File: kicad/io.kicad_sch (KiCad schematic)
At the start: 20 parts, among them J4 DE9_Plug_MountingHoles, J5 DB25_Receptacle_MountingHoles, U29 6522, U30 6551, U31 6551, U32 MAX232, U34 24LC256, X2 ACO-1.8432MHz-A

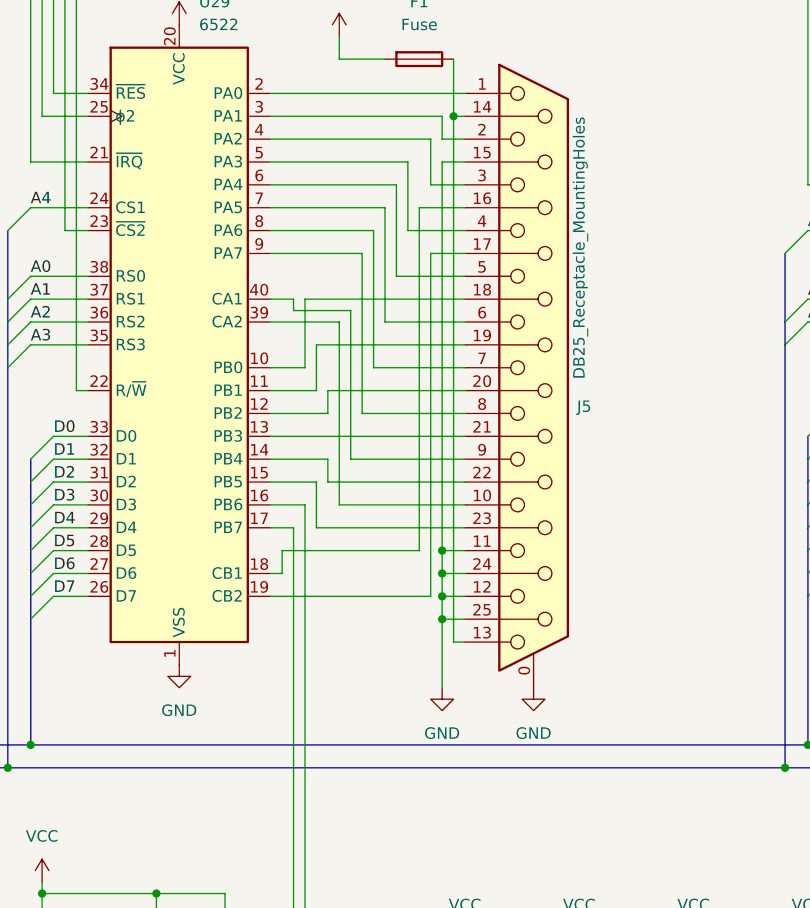
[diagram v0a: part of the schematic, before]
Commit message: Bugfixes, start routing
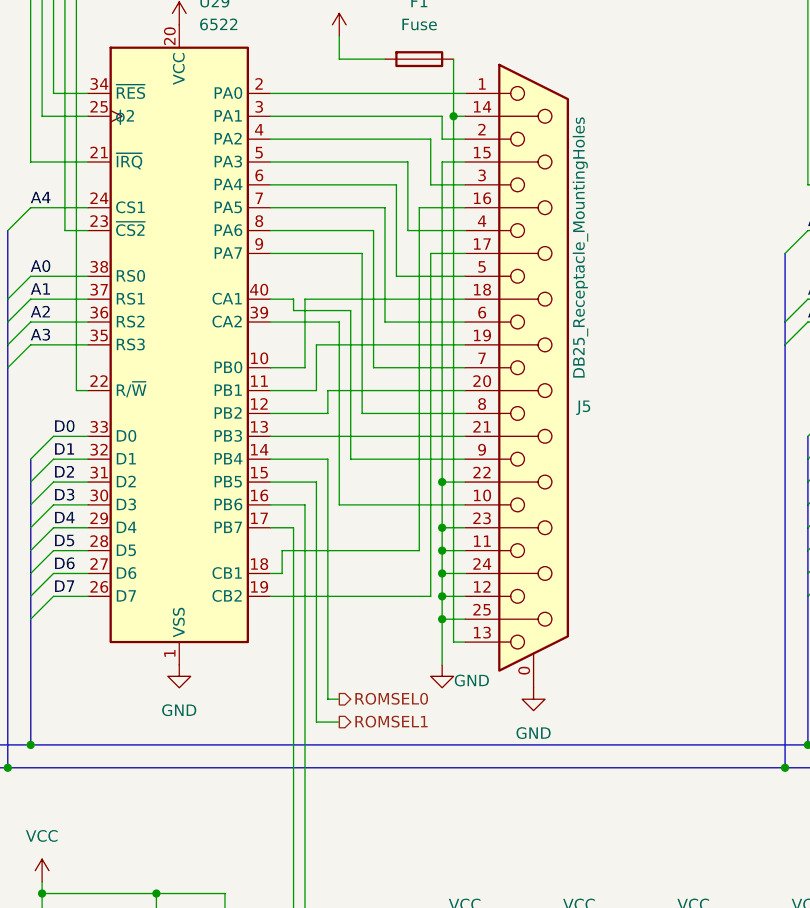
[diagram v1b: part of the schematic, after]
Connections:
- net GND: now also J5.22 (P22), J5.23 (P23)
- net ROMSEL0: now reaches U29.14 (PB4)
- net ROMSEL0: no longer J5.22 (P22)
- net ROMSEL1: now reaches U29.15 (PB5)
- net ROMSEL1: no longer J5.23 (P23)
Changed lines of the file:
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@@
 	)
 	(junction
+		(at 80.01 97.79)
+		(diameter 0)
+		(color 0 0 0 0)
+	)
+	(junction
 		(at 242.57 26.67)
 		(diameter 0)
@@
 	)
 	(junction
+		(at 80.01 92.71)
+		(diameter 0)
+		(color 0 0 0 0)
+	)
+	(junction
 		(at 35.56 138.43)
 		(diameter 0)
@@
 	(wire
 		(pts
+			(xy 80.01 97.79) (xy 80.01 92.71)
+		)
+		(stroke
+			(width 0)
+			(type default)
+		)
+	)
+	(wire
+		(pts
 			(xy 137.16 114.3) (xy 148.59 114.3)
 		)
@@
 	(wire
 		(pts
-			(xy 66.04 92.71) (xy 66.04 97.79)
+			(xy 66.04 92.71) (xy 66.04 119.38)
 		)
 		(stroke
@@
 	(wire
 		(pts
+			(xy 80.01 97.79) (xy 82.55 97.79)
+		)
+		(stroke
+			(width 0)
+			(type default)
+		)
+	)
+	(wire
+		(pts
 			(xy 35.56 162.56) (xy 24.13 162.56)
 		)
@@
 	(wire
 		(pts
+			(xy 80.01 92.71) (xy 82.55 92.71)
+		)
+		(stroke
+			(width 0)
+			(type default)
+		)
+	)
+	(wire
+		(pts
 			(xy 63.5 73.66) (xy 69.85 73.66)
 		)
@@
 		)
 	)
+	(wire
+		(pts
+			(xy 66.04 119.38) (xy 68.58 119.38)
+		)
+		(stroke
+			(width 0)
+			(type default)
+		)
+	)
 	(bus
 		(pts
@@
 	(wire
 		(pts
+			(xy 67.31 116.84) (xy 68.58 116.84)
+		)
+		(stroke
+			(width 0)
+			(type default)
+		)
+	)
+	(wire
+		(pts
 			(xy 265.43 128.27) (xy 262.89 128.27)
 		)
@@
 	(wire
 		(pts
-			(xy 66.04 97.79) (xy 82.55 97.79)
-		)
-		(stroke
-			(width 0)
-			(type default)
-		)
-	)
-	(wire
-		(pts
 			(xy 255.27 154.94) (xy 265.43 154.94)
 		)
@@
 		)
 	)
-	(wire
-		(pts
-			(xy 67.31 92.71) (xy 82.55 92.71)
-		)
-		(stroke
-			(width 0)
-			(type default)
-		)
-	)
 	(bus
 		(pts
@@
 	(wire
 		(pts
-			(xy 80.01 115.57) (xy 80.01 107.95)
+			(xy 80.01 113.03) (xy 80.01 107.95)
 		)
 		(stroke
@@
 	(wire
 		(pts
+			(xy 80.01 92.71) (xy 80.01 57.15)
+		)
+		(stroke
+			(width 0)
+			(type default)
+		)
+	)
+	(wire
+		(pts
 			(xy 209.55 104.14) (xy 222.25 104.14)
 		)
@@
 	(wire
 		(pts
-			(xy 80.01 100.33) (xy 80.01 57.15)
+			(xy 80.01 100.33) (xy 80.01 97.79)
 		)
 		(stroke
@@
 		)
 	)
-	(bus
+	(wire
 		(pts
-			(xy 34.29 95.25) (xy 34.29 97.79)
+			(xy 67.31 90.17) (xy 67.31 116.84)
 		)
 		(stroke
@@
 		)
 	)
-	(wire
+	(bus
 		(pts
-			(xy 67.31 90.17) (xy 67.31 92.71)
+			(xy 34.29 95.25) (xy 34.29 97.79)
 		)
 		(stroke
@@
 		)
 	)
+	(hierarchical_label "ROMSEL1"
+		(shape output)
+		(at 68.58 119.38 0)
+		(fields_autoplaced yes)
+		(effects
+			(font
+				(size 1.27 1.27)
+			)
+			(justify left)
+		)
+	)
+	(hierarchical_label "ROMSEL0"
+		(shape output)
+		(at 68.58 116.84 0)
+		(fields_autoplaced yes)
+		(effects
+			(font
+				(size 1.27 1.27)
+			)
+			(justify left)
+		)
+	)
 	(hierarchical_label "R{slash}W"
 		(shape input)
@@
 	(symbol
 		(lib_id "power:GND")
-		(at 80.01 115.57 0)
+		(at 80.01 113.03 0)
 		(unit 1)
 		(exclude_from_sim no)
@@
 		(on_board yes)
 		(dnp no)
-		(fields_autoplaced yes)
 		(property "Reference" "#PWR074"
-			(at 80.01 121.92 0)
+			(at 80.01 119.38 0)
 			(effects
 				(font
@@
 		)
 		(property "Value" "GND"
-			(at 80.01 120.65 0)
+			(at 83.312 114.808 0)
 			(effects
 				(font
@@
 		)
 		(property "Footprint" ""
-			(at 80.01 115.57 0)
+			(at 80.01 113.03 0)
 			(effects
 				(font
@@
 		)
 		(property "Datasheet" ""
-			(at 80.01 115.57 0)
+			(at 80.01 113.03 0)
 			(effects
 				(font
@@
 		)
 		(property "Description" "Power symbol creates a global label with name \"GND\" , ground"
-			(at 80.01 115.57 0)
+			(at 80.01 113.03 0)
 			(effects
 				(font
